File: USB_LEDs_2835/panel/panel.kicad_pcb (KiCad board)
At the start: 2 copper layers, 105.9 x 100 mm, 280 parts, among them U1 MT9284_1, U2 JL8022W-L, U3 74LVC1G04

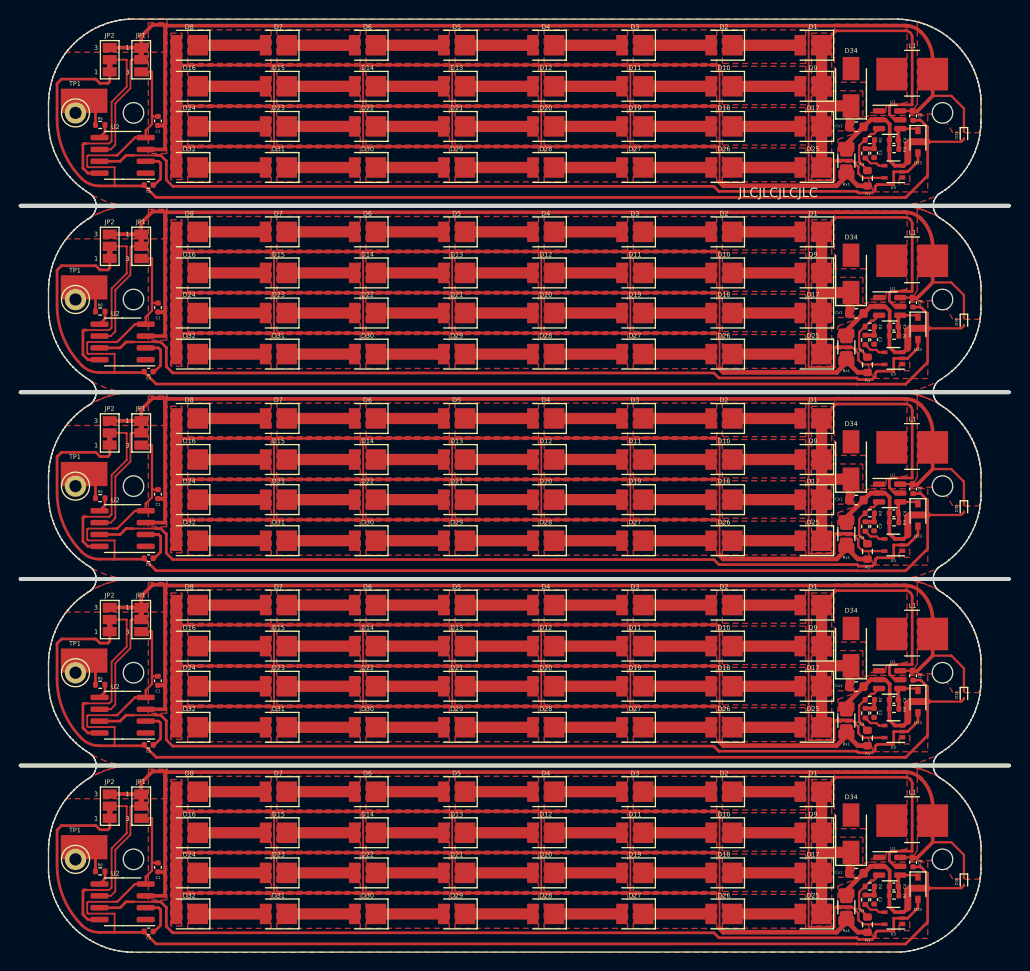
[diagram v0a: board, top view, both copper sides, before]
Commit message: Add files via upload
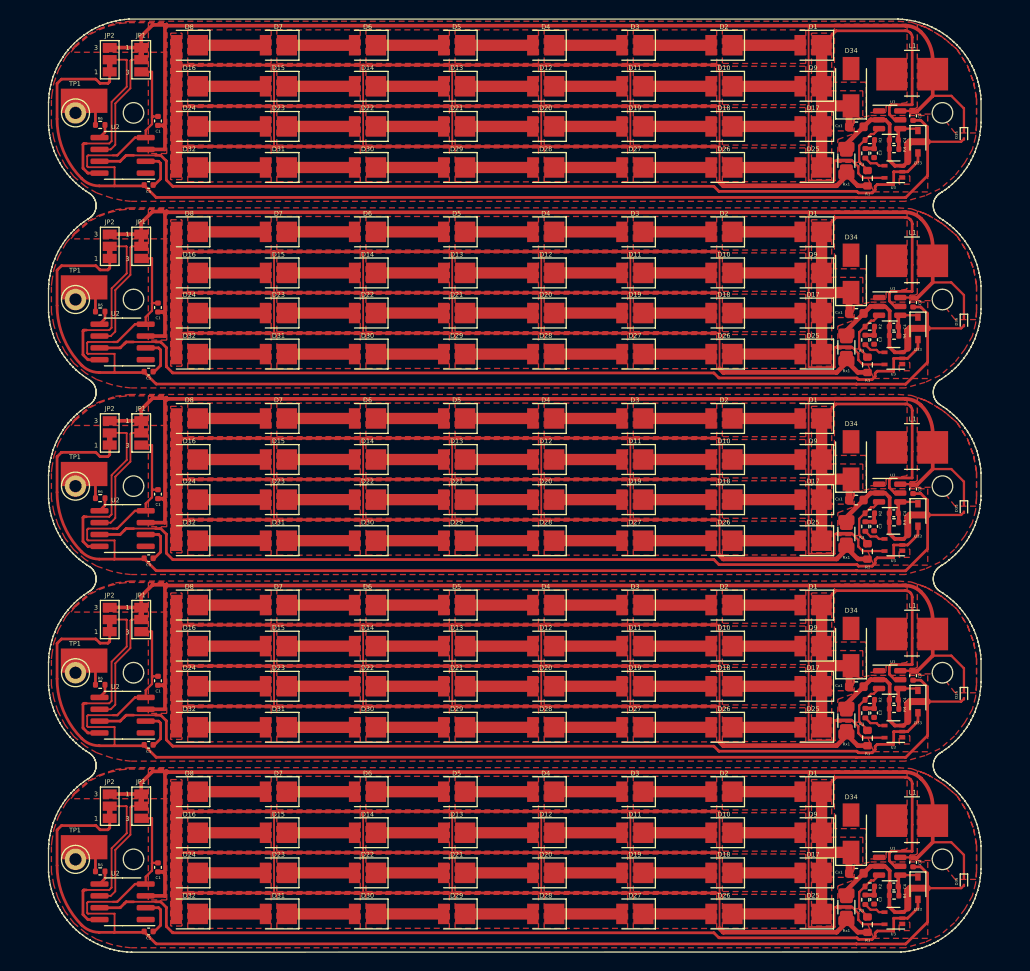
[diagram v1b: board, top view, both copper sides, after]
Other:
- board size 105.9 x 100 mm -> 99.9 x 100 mm
- board text removed: "JLCJLCJLCJLC"
